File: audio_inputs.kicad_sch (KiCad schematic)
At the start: 12 parts, among them J2 AFBR-2624Z, U4 DIR9001PW, Y1 12.288 MHz

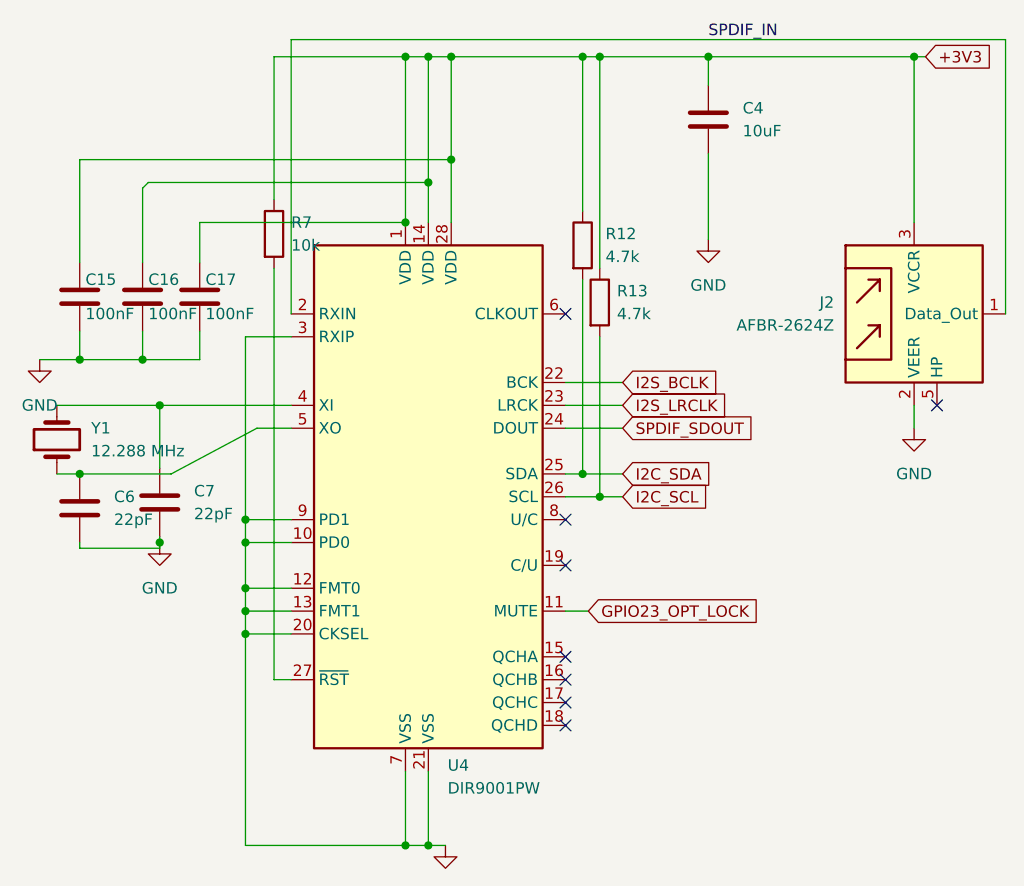
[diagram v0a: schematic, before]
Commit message: Fixed some connections and global labels
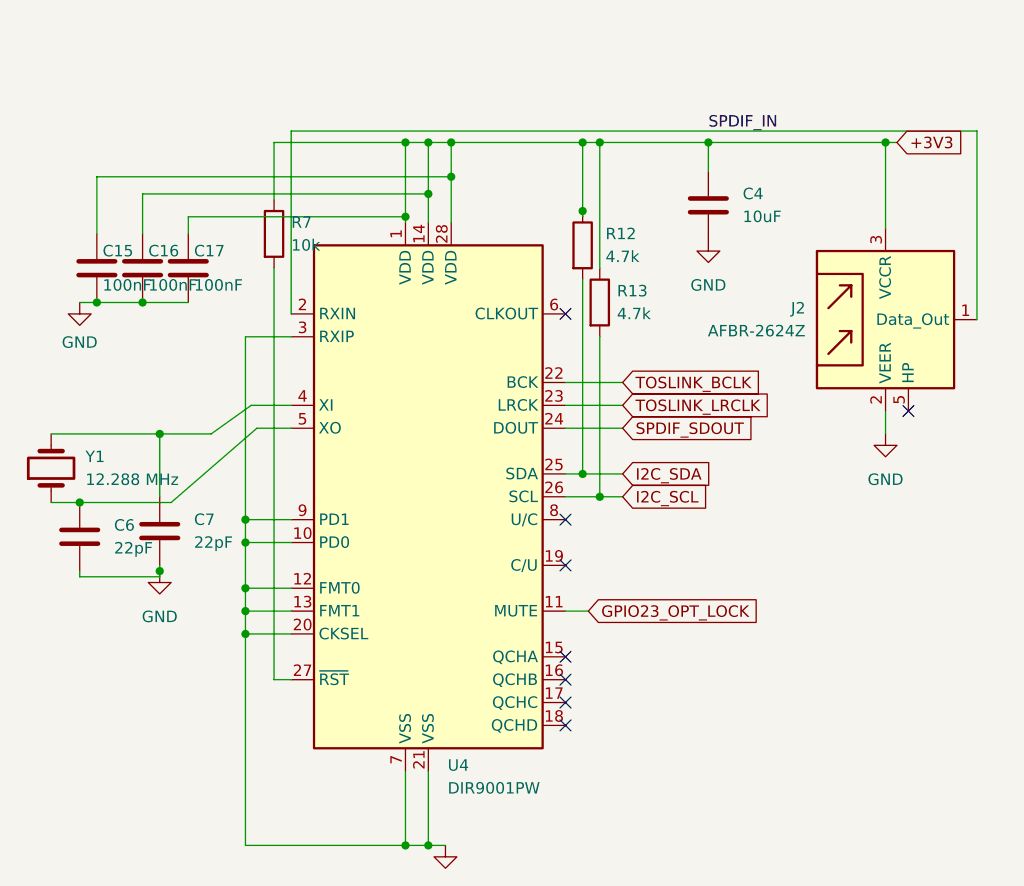
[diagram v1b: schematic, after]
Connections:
- net I2S_BCLK renamed TOSLINK_BCLK
- net I2S_LRCLK renamed TOSLINK_LRCLK
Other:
- moved on the sheet: C15, C16, C17, C4, C6, C7, J2, Y1
